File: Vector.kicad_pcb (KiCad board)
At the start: 2 copper layers, 54.6 x 52.7 mm, 37 parts, among them J1 Conn_01x06_Female, J2 Barrel_Jack_Switch, Q1 BC547, Q2 BC547, Q3 BC547, Q4 BC547

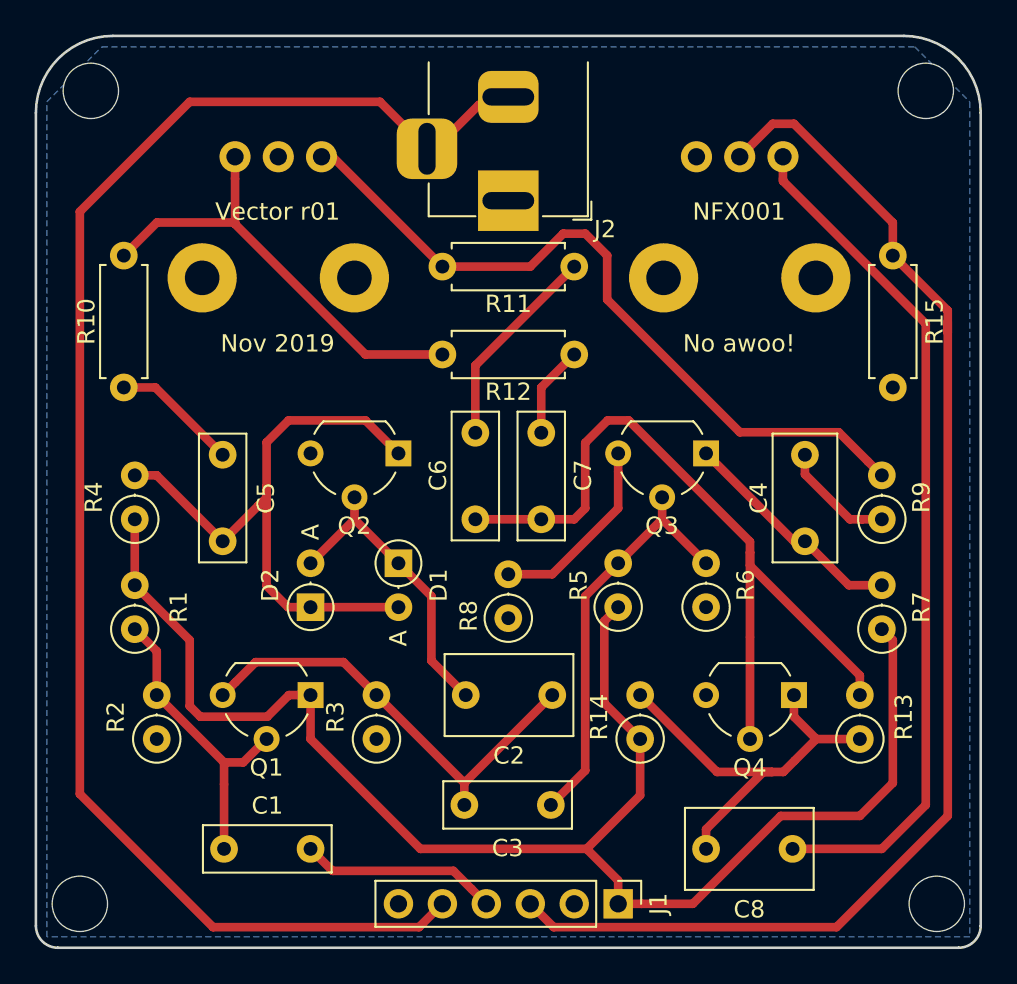
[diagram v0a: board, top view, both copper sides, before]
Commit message: Migrate to KiCAD 6
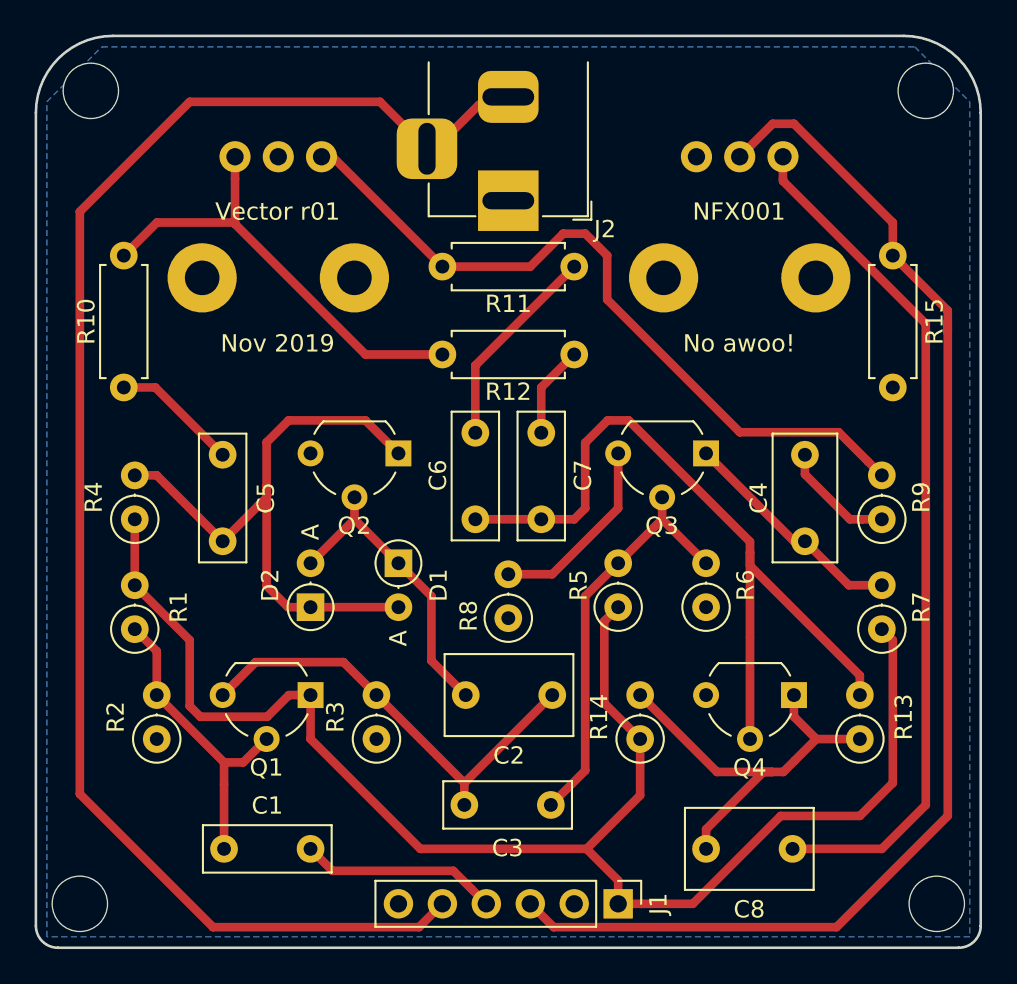
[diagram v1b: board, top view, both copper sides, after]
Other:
- net class Default removed
